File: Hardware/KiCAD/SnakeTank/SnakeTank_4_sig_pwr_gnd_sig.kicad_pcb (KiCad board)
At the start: 4 copper layers, 80.5 x 36.6 mm, 51 parts, among them J1 Conn_01x12, J2 USB_C_Receptacle_USB2.0_16P, J3 RJ45, Q1 L8050QLT1G, Q2 L8050QLT1G, U1 LP2985-3.3, U2 ESP32-S3-WROOM-1-N8, U4 FT231XS

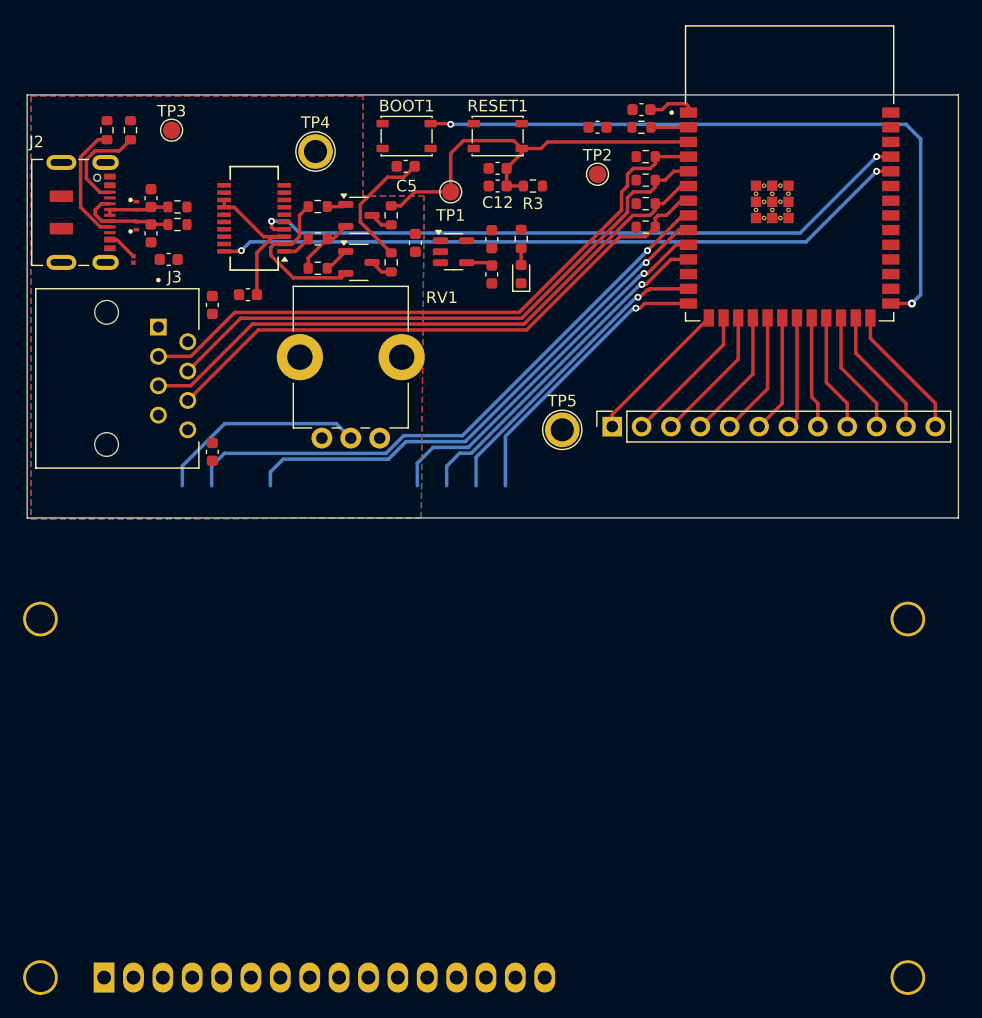
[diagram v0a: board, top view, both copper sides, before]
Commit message: layout Rough
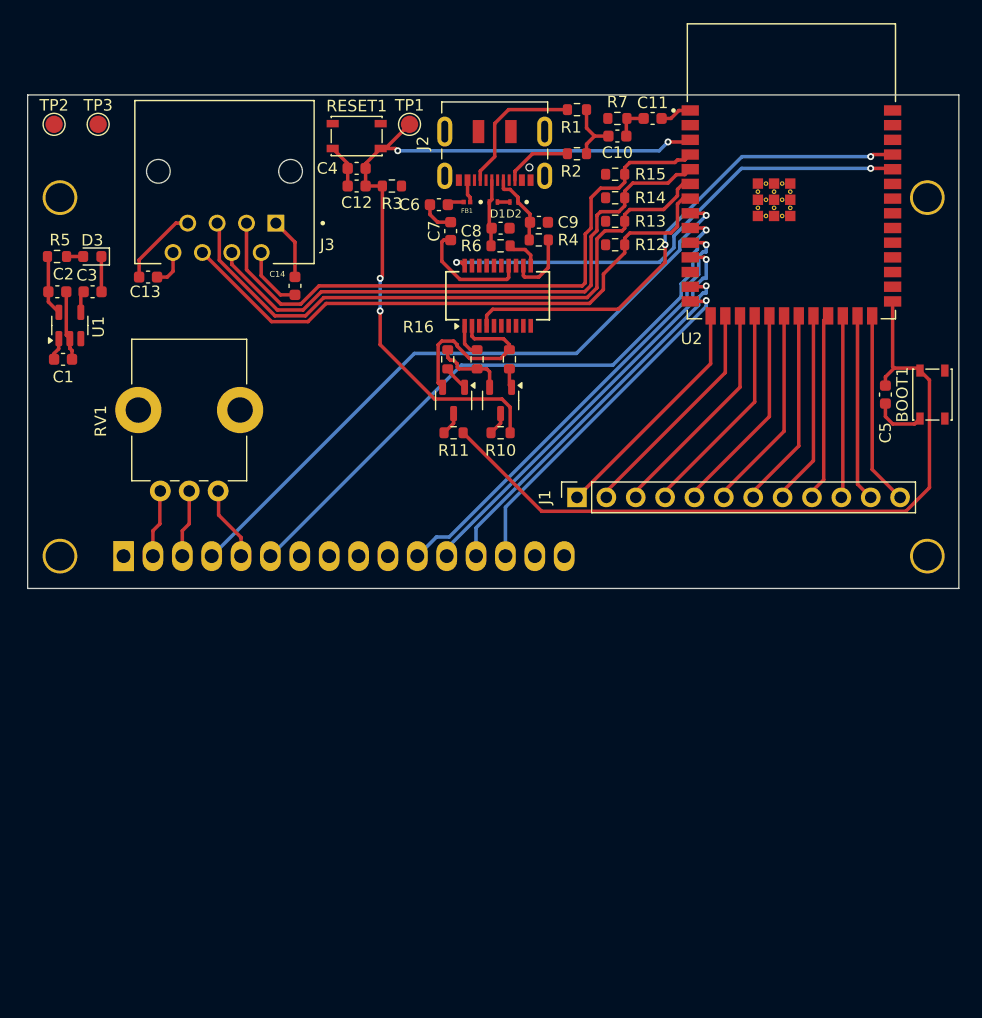
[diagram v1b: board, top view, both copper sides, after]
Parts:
- removed TP4, TP5: GND_TP, TestPoint:TestPoint_Plated_Hole_D2.0mm
- moved BOOT1 50.7 mm to (96.3, 50.0), turned to 90 degrees
- moved TP2 47.2 mm to (20.3, 26.7)
- moved C5 45.9 mm to (92.2, 50.0), turned to -90 degrees
- moved R1 40.7 mm to (65.5, 25.4), turned to 0 degrees
- moved R5 40.2 mm to (20.6, 38.1), turned to 0 degrees
- moved R2 38.7 mm to (65.5, 29.2), turned to 0 degrees
- moved C2 37.8 mm to (20.6, 41.1), turned to 0 degrees
- moved D3 37.1 mm to (23.6, 38.1), turned to 180 degrees
- moved J2 36.8 mm to (58.4, 28.4), turned to 180 degrees
- moved DS1 36.5 mm to (26.3, 64.0)
- moved C3 34.6 mm to (23.6, 41.1), turned to 0 degrees
- moved U1 33.8 mm to (21.7, 44.1), turned to 90 degrees
- moved C9 33.6 mm to (62.2, 35.1), turned to 0 degrees
- moved D2 32.7 mm to (60.1, 33.4), turned to 180 degrees
- moved C1 32.1 mm to (21.1, 47.0), turned to 0 degrees
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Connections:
- net /USBN renamed Net-(U4-USBDM)
- net /USBP renamed Net-(U4-USBDP)
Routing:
- net GND: track 4.21 -> 45.1 mm
- net /CHIP_PU: track 36.4 -> 65.3 mm, vias 0 -> 4
- net +5V: track 0.00 -> 21.6 mm
- net /FDTI_UART_TX: track 60.5 -> 42.5 mm
- net /FTDI_UART_RX: track 58.4 -> 43.2 mm
- net Net-(DS1-VO): track 18.3 -> 5.88 mm
- net +3.3V: track 0.00 -> 8.23 mm
- net IO3: track 12.9 -> 20.6 mm
- net IO9: track 11.8 -> 19.3 mm
- net IO10: track 11.3 -> 18.8 mm
- net IO46: track 12.3 -> 19.8 mm
- net IO12: track 10.2 -> 17.7 mm
- net IO13: track 9.70 -> 17.2 mm
- net IO11: track 10.7 -> 18.2 mm
- net IO14: track 9.61 -> 16.6 mm
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- removed copper zone on B.Cu, net +5V
- removed copper zone on F.Cu, net +5V
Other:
- board size 80.5 x 36.6 mm -> 80.5 x 42.7 mm
